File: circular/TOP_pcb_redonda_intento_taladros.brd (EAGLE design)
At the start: 65 x 65 mm, 9 parts, among them X1 DSB18b20

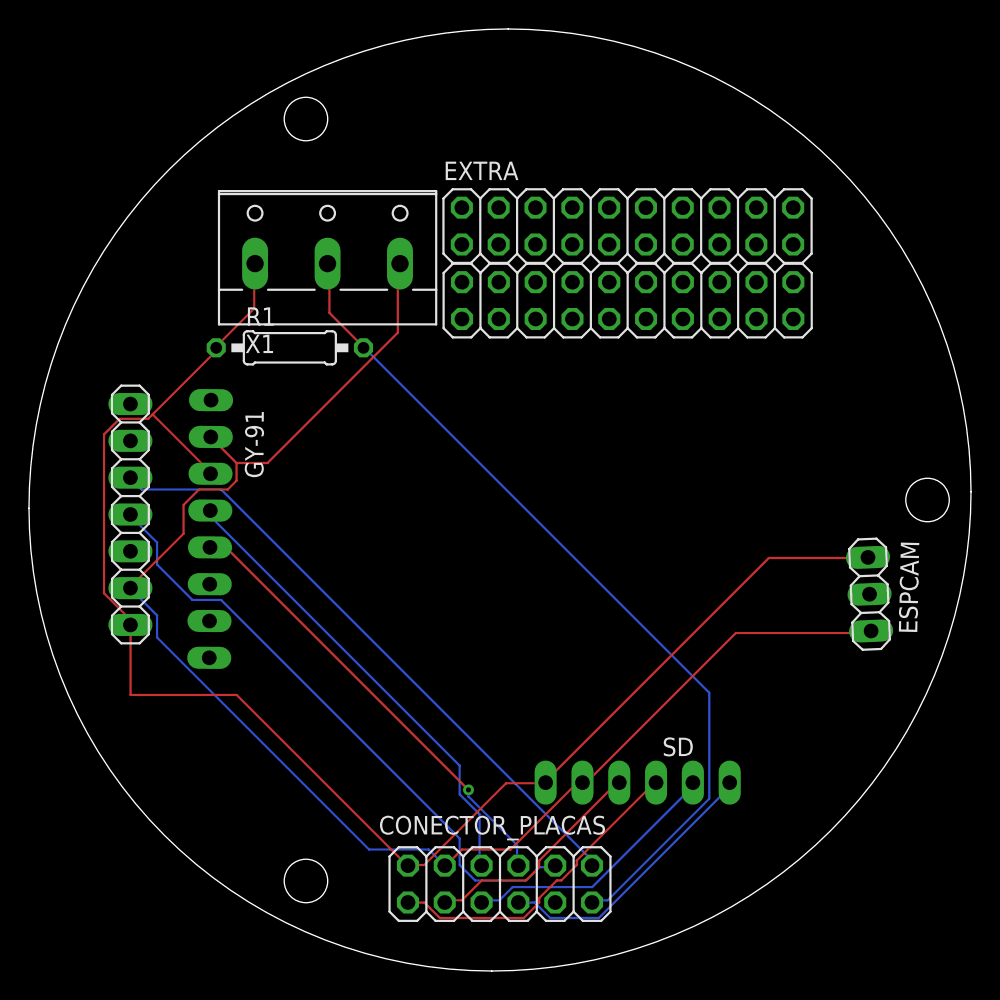
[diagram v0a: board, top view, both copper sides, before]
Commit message: Add files via upload
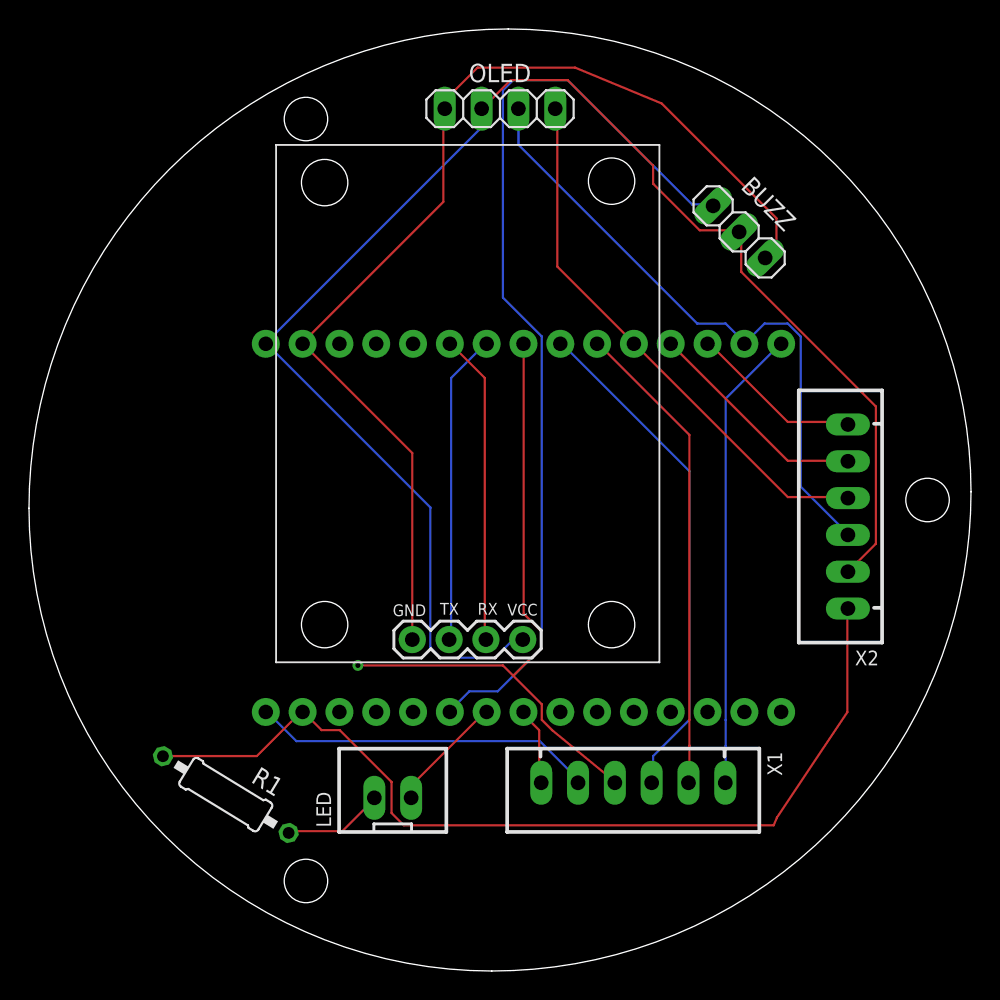
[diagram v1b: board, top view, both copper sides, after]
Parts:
- removed APC220: (no value), pinhead:1X07
- removed CONECTOR_PLACAS: (no value), pinhead:2X06
- removed ESPCAM: (no value), pinhead:1X03
- removed EXTRA, EXTRA2: (no value), pinhead:2X10
- removed GY-91: (no value), pinhead:1X08
- removed SD: (no value), pinhead:1X06
- added BUZZ: (no value), pinhead:1X03
- added GPS: U-BLOX-NEO6V2, u-blox neo-6m v2:U-BLOX-NEO6V2
- added LED: JST-XH-02-PIN-LONG-PAD, Rembrandt Electronics - JST XH Connectors v1-0:JST-XH-02-PACKAGE-LONG-PAD
- added OLED: (no value), pinhead:1X04
- added PLACA: ESP32DEVKITV1, ESP32-DEVKITV1:ESP32-DEVKITV1
- added X2: JST-XH-06-PIN-LONG-PAD, Rembrandt Electronics - JST XH Connectors v1-0:JST-XH-06-PACKAGE-LONG-PAD
- X1: value DSB18b20 -> JST-XH-06-PIN-LONG-PAD; device con-wago-500:W237-103 -> Rembrandt Electronics - JST XH Connectors v1-0:JST-XH-06-PACKAGE-LONG-PAD
- moved X1 42.7 mm to (41.7, 13.0), turned to 180 degrees
- moved R1 31.1 mm to (13.6, 12.2), turned to 148.6 degrees
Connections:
- new net GPS: BUZZ.3, GPS.GND, OLED.1, PLACA.GND@2
- new net N$12: LED.1, R1.1
- new net N$13: BUZZ.1, PLACA.D27
- new net N$14: PLACA.D23, X1.1
- new net N$15: PLACA.D19, X1.2
- new net N$16: PLACA.D18, X1.3
- new net N$17: PLACA.D5, X1.4
- net N$1: now also BUZZ.2, GPS.VCC, OLED.2, PLACA.3V3, X2.2; no longer APC220.2, CONECTOR_PLACAS.4, ESPCAM.3, GY-91.2, SD.5, X1.3
- net N$10: now also PLACA.D25, X1.6; no longer CONECTOR_PLACAS.1, SD.3
- net N$11: now also LED.2, PLACA.D26; no longer CONECTOR_PLACAS.3, SD.4
- net N$2: now also PLACA.GND@1, R1.2, X2.1; no longer CONECTOR_PLACAS.7, SD.1
- net N$3: now also PLACA.VIN, X1.5; no longer APC220.4, CONECTOR_PLACAS.10
- net N$4: now also OLED.3, PLACA.D22, X2.3; no longer APC220.5, CONECTOR_PLACAS.12
- net N$5: now also OLED.4, PLACA.D21, X2.4; no longer CONECTOR_PLACAS.6, GY-91.4
- net N$6: now also PLACA.D3, X2.5; no longer CONECTOR_PLACAS.8, GY-91.5
- net N$7: now also PLACA.D1, X2.6; no longer APC220.1, CONECTOR_PLACAS.2, ESPCAM.1, GY-91.3, R1.1, SD.6, X1.1
- net N$8: now also GPS.RX, PLACA.D16; no longer CONECTOR_PLACAS.11, R1.2, X1.2
- net N$9: now also GPS.TX, PLACA.D17; no longer CONECTOR_PLACAS.5, SD.2
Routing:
- net N$7: track 106.5 -> 12.1 mm
- net GPS: track 0.00 -> 75.0 mm
- net N$13: track 0.00 -> 66.2 mm
- net N$17: track 0.00 -> 45.8 mm, vias 0 -> 1
- net N$2: track 19.1 -> 64.4 mm
- net N$8: track 59.0 -> 21.5 mm
- net N$16: track 0.00 -> 35.1 mm
- net N$15: track 0.00 -> 33.0 mm
- net N$14: track 0.00 -> 31.9 mm
- net N$3: track 42.2 -> 23.9 mm
- net N$10: track 21.8 -> 5.60 mm
- net N$6: track 31.5 -> 15.6 mm, vias 1 -> 0
- net N$11: track 15.9 -> 8.18 mm
- net N$12: track 0.00 -> 6.96 mm
- net N$5: track 32.3 -> 37.6 mm
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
